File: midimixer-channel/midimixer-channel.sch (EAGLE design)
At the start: 114 parts, among them IC1 74LS595D, IC2 74LS595D, IC3 74LS595D, IC4 74165D, IC5 74165D, U1 LM1117IMPX-3.3/NOPB

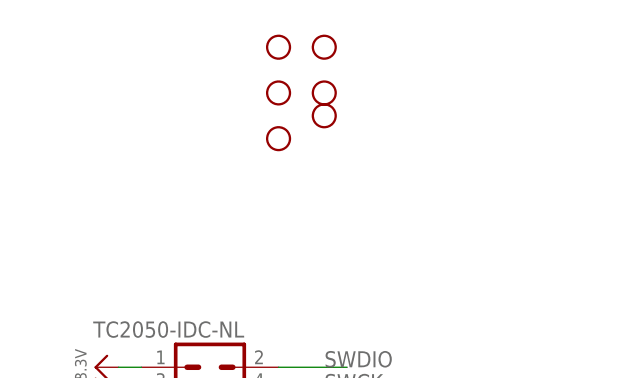
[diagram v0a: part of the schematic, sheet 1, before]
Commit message: wip
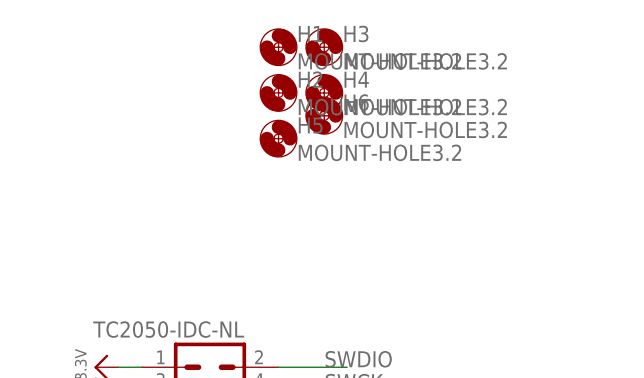
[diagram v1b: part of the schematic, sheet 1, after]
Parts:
- H1, H2, H3, H4, H5, H6: value STAND-OFF -> MOUNT-HOLE3.2; device SparkFun-Electromechanical:STAND-OFF -> holes:MOUNT-HOLE3.2
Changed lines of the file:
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@@
 <part name="U$76" library="microbuilder" deviceset="GND" device=""/>
 <part name="U$77" library="microbuilder" deviceset="3.3V" device=""/>
-<part name="H3" library="SparkFun-Electromechanical" deviceset="STAND-OFF" device=""/>
-<part name="H4" library="SparkFun-Electromechanical" deviceset="STAND-OFF" device=""/>
-<part name="H1" library="SparkFun-Electromechanical" deviceset="STAND-OFF" device=""/>
-<part name="H2" library="SparkFun-Electromechanical" deviceset="STAND-OFF" device=""/>
+<part name="H3" library="holes" deviceset="MOUNT-HOLE" device="3.2"/>
+<part name="H4" library="holes" deviceset="MOUNT-HOLE" device="3.2"/>
+<part name="H1" library="holes" deviceset="MOUNT-HOLE" device="3.2"/>
+<part name="H2" library="holes" deviceset="MOUNT-HOLE" device="3.2"/>
 <part name="U$78" library="microbuilder" deviceset="GND" device=""/>
 <part name="U$79" library="microbuilder" deviceset="GND" device=""/>
@@
 <part name="R38" library="microbuilder" deviceset="RESISTOR" device="_0603" value="10k"/>
 <part name="U$47" library="microbuilder" deviceset="3.3V" device=""/>
-<part name="H5" library="SparkFun-Electromechanical" deviceset="STAND-OFF" device=""/>
-<part name="H6" library="SparkFun-Electromechanical" deviceset="STAND-OFF" device=""/>
+<part name="H5" library="holes" deviceset="MOUNT-HOLE" device="3.2"/>
+<part name="H6" library="holes" deviceset="MOUNT-HOLE" device="3.2"/>
 <part name="POT2" library="keves" deviceset="POTENTIOMETER" device="PTV09A_VERTICAL"/>
 <part name="POT7" library="keves" deviceset="POTENTIOMETER" device="PTV09A_VERTICAL"/>
